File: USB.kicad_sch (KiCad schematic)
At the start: 7 parts, among them J6 Conn_01x06

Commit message: Release candidate
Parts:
- R22, R23: footprint Resistor_SMD:R_0805_2012Metric_Pad1.20x1.40mm_HandSolder -> Resistor_SMD:R_0603_1608Metric_Pad0.98x0.95mm_HandSolder; MPN RC0805JR-0751RL -> RC0603JR-0751RL
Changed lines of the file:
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@@
 (kicad_sch
-	(version 20260101)
+	(version 20260306)
 	(generator "eeschema")
 	(generator_version "10.0")
@@
 			)
 		)
-		(property "Footprint" "Resistor_SMD:R_0805_2012Metric_Pad1.20x1.40mm_HandSolder"
+		(property "Footprint" "Resistor_SMD:R_0603_1608Metric_Pad0.98x0.95mm_HandSolder"
 			(at 121.92 97.028 90)
 			(hide yes)
@@
 			)
 		)
-		(property "MPN" "RC0805JR-0751RL"
+		(property "MPN" "RC0603JR-0751RL"
 			(at 121.92 95.25 90)
 			(hide yes)
@@
 			)
 		)
-		(property "Footprint" "Resistor_SMD:R_0805_2012Metric_Pad1.20x1.40mm_HandSolder"
+		(property "Footprint" "Resistor_SMD:R_0603_1608Metric_Pad0.98x0.95mm_HandSolder"
 			(at 113.03 99.568 90)
 			(hide yes)
@@
 			)
 		)
-		(property "MPN" "RC0805JR-0751RL"
+		(property "MPN" "RC0603JR-0751RL"
 			(at 113.03 97.79 90)
 			(hide yes)

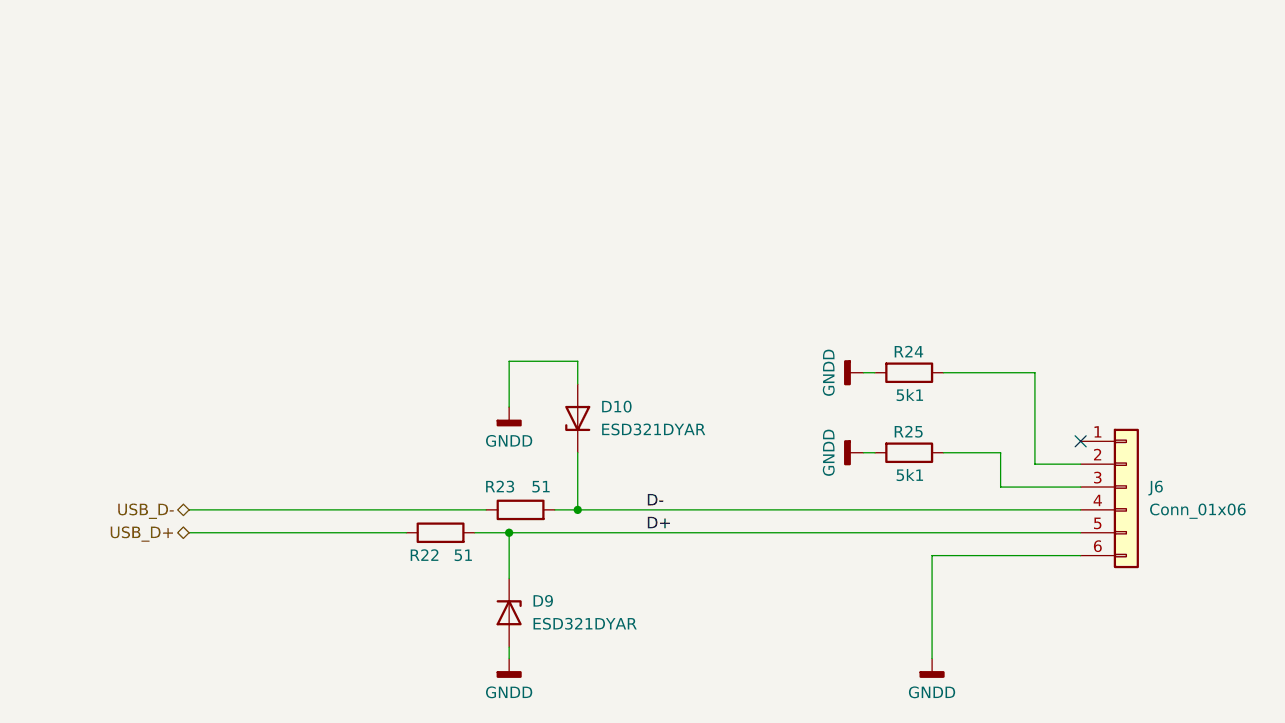
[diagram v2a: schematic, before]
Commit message: Proproduction version
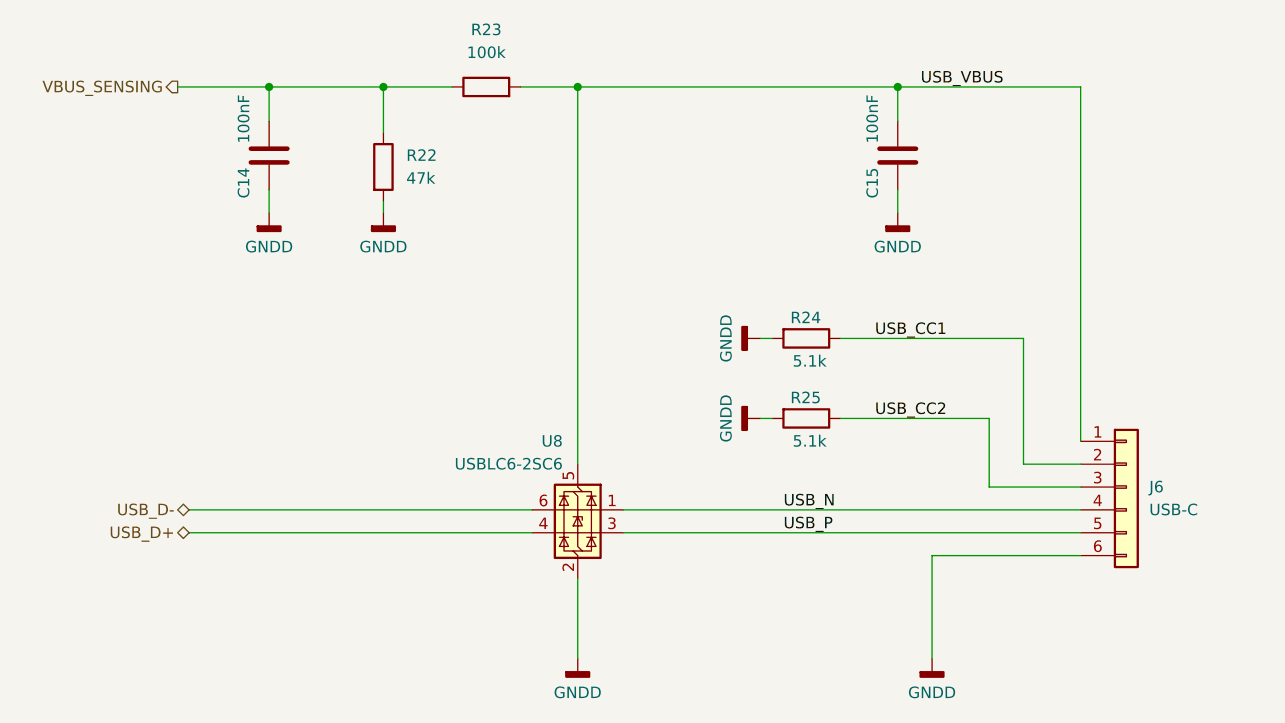
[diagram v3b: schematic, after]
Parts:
- removed D10, D9: ESD321DYAR, Diode_SMD:D_SOD-523, symbol Diode:ESD5Zxx
- added C14, C15: 100nF, Capacitor_SMD:C_0805_2012Metric_Pad1.18x1.45mm_HandSolder, symbol Device:C
- added U8: USBLC6-2SC6, Package_TO_SOT_SMD:SOT-23-6, symbol Power_Protection:USBLC6-2SC6
- J6: value Conn_01x06 -> USB-C
- R22: value 51 -> 47k; footprint Resistor_SMD:R_0603_1608Metric_Pad0.98x0.95mm_HandSolder -> Resistor_SMD:R_0805_2012Metric_Pad1.20x1.40mm_HandSolder; MPN RC0603JR-0751RL -> RC0805JR-0747KL
- R23: value 51 -> 100k; footprint Resistor_SMD:R_0603_1608Metric_Pad0.98x0.95mm_HandSolder -> Resistor_SMD:R_0805_2012Metric_Pad1.20x1.40mm_HandSolder; MPN RC0603JR-0751RL -> RC0805JR-07100KL
- R24, R25: value 5k1 -> 5.1k
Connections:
- net GNDD: now also R22.2, C14.1, C15.1, U8.2 (GND)
- net USB_D+: now also U8.4 (I/O2); no longer R22.1
- net USB_D-: now also U8.6 (I/O1); no longer R23.1
- net USB_CC2: now reaches J6.3 (Pin_3), R25.1
- net USB_CC1: now reaches J6.2 (Pin_2), R24.1
- net USB_VBUS: now reaches J6.1 (Pin_1)
- net USB_VBUS: now also R23.2, C15.2, U8.5 (VBUS)
- net D+ renamed USB_P
- net USB_P: now also U8.3 (I/O2); no longer R22.2
- net D- renamed USB_N
- net USB_N: now also U8.1 (I/O1); no longer R23.2
- new net VBUS_SENSING: C14.2, R22.1, R23.1
- no-connect marks 1 -> 0
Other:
- moved on the sheet: R24, R25
